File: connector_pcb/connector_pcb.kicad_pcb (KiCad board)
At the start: 2 copper layers, 17 x 9 mm, 2 parts, among them IC1 WSEN-PDUS_2513130810402, J7 Conn_02x04_Top_Bottom

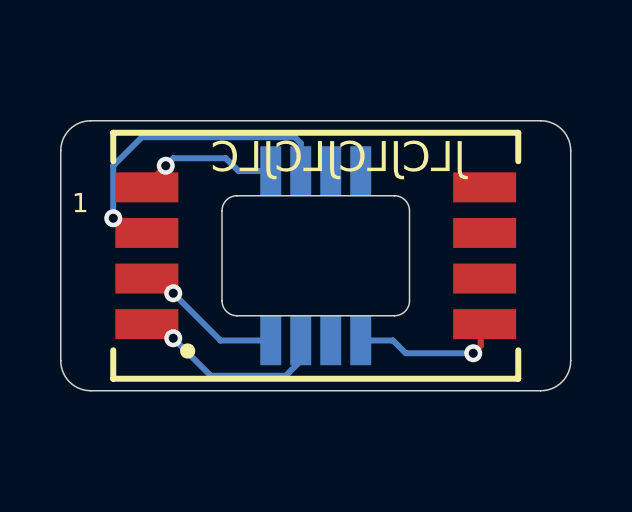
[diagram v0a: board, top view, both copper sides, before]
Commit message: some changes according to manu, added connector board
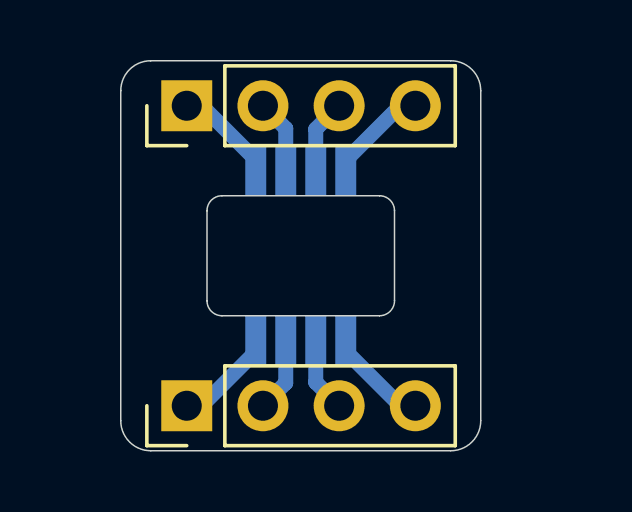
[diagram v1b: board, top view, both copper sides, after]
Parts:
- removed IC1: WSEN-PDUS_2513130810402, fancyfins:WE-FP-PDUS-1V
- added J1: Conn_01x04_Pin, Connector_PinHeader_2.54mm:PinHeader_1x04_P2.54mm_Vertical, F.Cu at (95.7, 60.0)
- added J2: ~, Connector_PinHeader_2.54mm:PinHeader_1x04_P2.54mm_Vertical, F.Cu at (95.7, 70.0)
- moved J7 0.50 mm to (99.5, 65.0)
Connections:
- J7 pad 3: unconnected-(J7-Pin_3-Pad3) -> Net-(J1-Pin_3)
- J7 pad 4: unconnected-(J7-Pin_4-Pad4) -> Net-(J1-Pin_4)
- J7 pad 7: unconnected-(J7-Pin_7-Pad7) -> Net-(J2-Pin_3)
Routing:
- net Net-(J1-Pin_2): track 11.2 -> 2.49 mm, vias 1 -> 0
- net Net-(J2-Pin_2): track 6.72 -> 2.49 mm, vias 1 -> 0
- net Net-(J1-Pin_4): track 0.00 -> 3.43 mm
- net Net-(J2-Pin_3): track 0.00 -> 2.50 mm
- net Net-(J1-Pin_3): track 0.00 -> 2.50 mm
- net Net-(J2-Pin_4): track 5.05 -> 3.43 mm, vias 1 -> 0
- net Net-(J1-Pin_1): track 5.00 -> 3.42 mm, vias 1 -> 0
- net Net-(J2-Pin_1): track 4.99 -> 3.42 mm, vias 1 -> 0
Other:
- board size 17 x 9 mm -> 12 x 13 mm
- board text removed: "HP UP"
- board text removed: "JLCJLCJLCJLC"
